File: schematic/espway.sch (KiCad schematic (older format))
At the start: 28 parts, among them J1 CONN_01X02, J2 CONN_01X02, J3 CONN_01X04_MALE, SW1 SW_Push, U1 DRV8835, U2 LM1117-3.3, U3 ESP-12E, U4 LSM6DS3

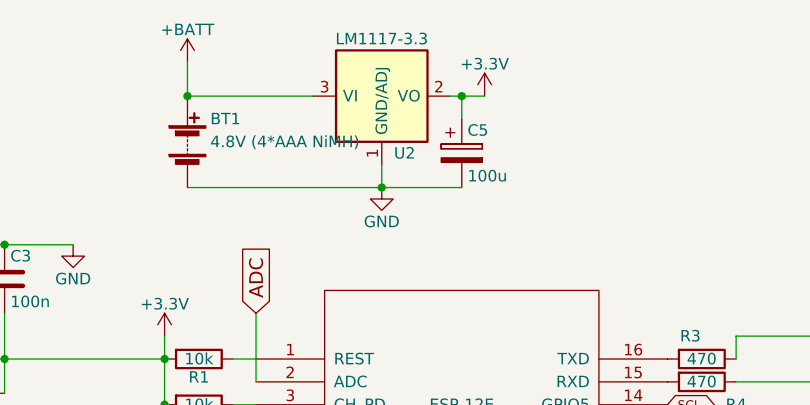
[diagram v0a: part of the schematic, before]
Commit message: Schematic and PCB update
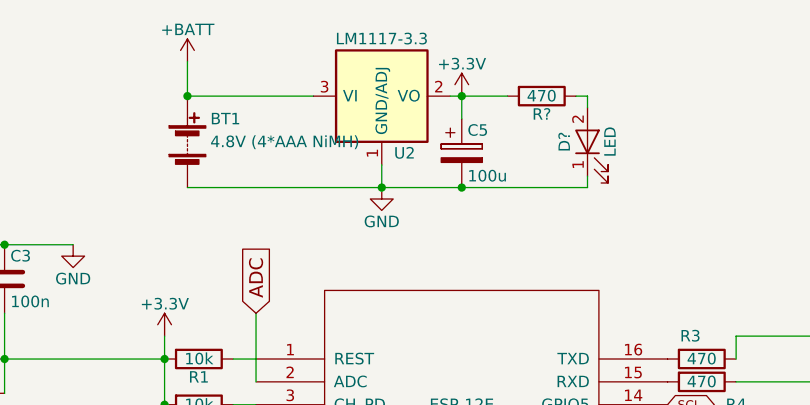
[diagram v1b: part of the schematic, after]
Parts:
- added D?: LED, symbol LED
- added R?: 470, symbol R
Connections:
- net +3V3: now also R?.2
- net GND: now also D?.1 (K)
- new net: D?.2 (A), R?.1
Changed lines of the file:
@@
 L +3.3V #PWR07
 U 1 1 59B82E61
-P 6300 1200
-F 0 "#PWR07" H 6300 1050 50  0001 C CNN
-F 1 "+3.3V" H 6300 1340 50  0000 C CNN
-F 2 "" H 6300 1200 50  0001 C CNN
-F 3 "" H 6300 1200 50  0001 C CNN
-	1    6300 1200
+P 6200 1200
+F 0 "#PWR07" H 6200 1050 50  0001 C CNN
+F 1 "+3.3V" H 6200 1340 50  0000 C CNN
+F 2 "" H 6200 1200 50  0001 C CNN
+F 3 "" H 6200 1200 50  0001 C CNN
+	1    6200 1200
 	1    0    0    -1
 $EndComp
@@
 	5850 1600 5850 1500
 Wire Wire Line
-	6300 1200 6150 1200
-Wire Wire Line
 	8250 5650 8250 5550
 Wire Wire Line
@@
 Wire Wire Line
 	6200 1300 6200 1200
-Connection ~ 6200 1200
-Wire Wire Line
-	5000 1600 6200 1600
+Wire Wire Line
+	5000 1600 6750 1600
 Wire Wire Line
 	2500 1850 4500 1850
@@
 Wire Wire Line
 	2750 2850 2750 2800
+$Comp
+L R R?
+U 1 1 59BE998C
+P 6550 1200
+F 0 "R?" V 6630 1200 50  0000 C CNN
+F 1 "470" V 6550 1200 50  0000 C CNN
+F 2 "" V 6480 1200 50  0001 C CNN
+F 3 "" H 6550 1200 50  0001 C CNN
+	1    6550 1200
+	0    1    1    0
+$EndComp
+$Comp
+L LED D?
+U 1 1 59BE99F7
+P 6750 1400
+F 0 "D?" H 6750 1500 50  0000 C CNN
+F 1 "LED" H 6750 1300 50  0000 C CNN
+F 2 "" H 6750 1400 50  0001 C CNN
+F 3 "" H 6750 1400 50  0001 C CNN
+	1    6750 1400
+	0    -1   -1   0
+$EndComp
+Wire Wire Line
+	6150 1200 6400 1200
+Connection ~ 6200 1200
+Wire Wire Line
+	6700 1200 6750 1200
+Wire Wire Line
+	6750 1200 6750 1250
+Wire Wire Line
+	6750 1600 6750 1550
+Connection ~ 6200 1600
 $EndSCHEMATC
